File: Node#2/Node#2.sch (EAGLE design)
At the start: 135 parts, among them IC1 TSL25911FN, J1 68712414522, Q1 BC847ALT1SMD, Q2 SI1308EDL-T1-GE3, Q3 FDN304PZ, U2 RV8564C3, U3 BLUENRG-232, U4 TPS63001DRCT, Y3 ECS-160-12-36-AGN-TR, Y4 NX2012SA-32.768K-STD-MUB-1

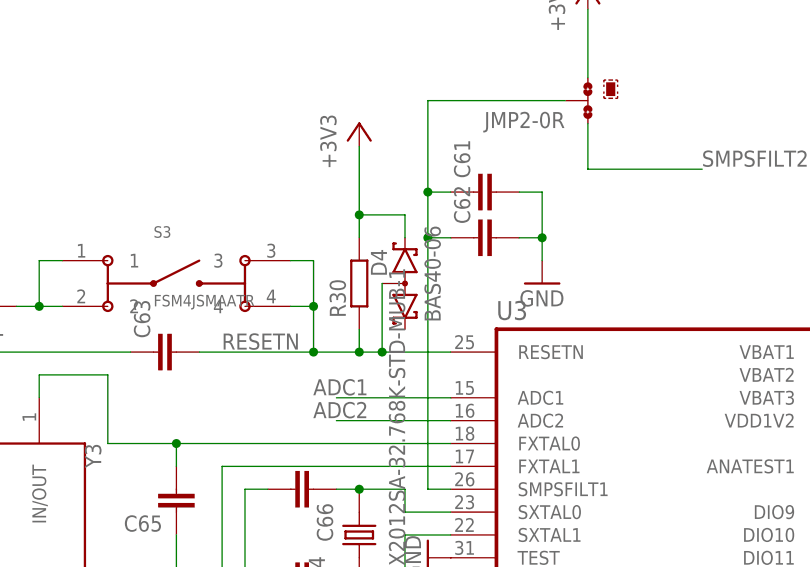
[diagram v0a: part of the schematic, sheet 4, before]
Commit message: display
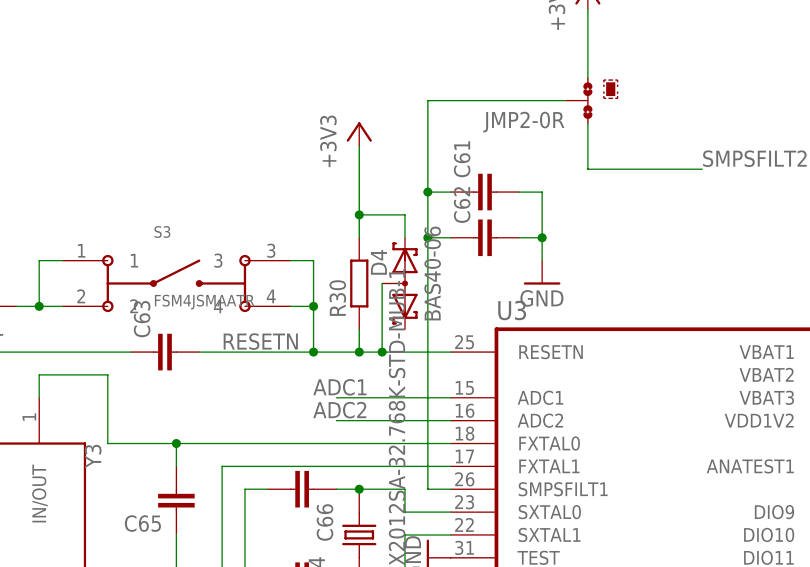
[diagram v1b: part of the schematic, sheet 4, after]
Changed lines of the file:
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@@
 <?xml version="1.0" encoding="utf-8"?>
 <!DOCTYPE eagle SYSTEM "eagle.dtd">
-<eagle version="9.3.0">
+<eagle version="9.2.1">
 <drawing>
 <settings>
@@
 <part name="C34" library="rcl" deviceset="C-EU" device="C0805" value="100n"/>
 <part name="LS1" library="BlueHome" deviceset="PS1720P02" device=""/>
-<part name="Q1" library="transistor-npn" library_urn="urn:adsk.eagle:library:398" deviceset="BC847*" device="SMD" package3d_urn="urn:adsk.eagle:package:28738/2" technology="ALT1"/>
+<part name="Q1" library="transistor-npn" library_urn="urn:adsk.eagle:library:398" deviceset="BC847*" device="SMD" package3d_urn="urn:adsk.eagle:package:28984/2" technology="ALT1"/>
 <part name="R4" library="rcl" deviceset="R-EU_" device="R0805"/>
 <part name="R6" library="rcl" deviceset="R-EU_" device="R0805"/>
